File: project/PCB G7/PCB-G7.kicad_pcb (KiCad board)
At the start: 2 copper layers, 56.5 x 88 mm, 28 parts, among them J13 jumper 1 2, J14 jumper 2 2, J15 stepper 1, J16 jumper 2 1, J17 stepper 1, J18 Barrel_Jack_Switch, J19 servomoteur, J2 Micro_SD_Card, J20 Oled, J9 jumper 1 1, U3 ESP32-S3-UNO, U4 R-78E5.0-1.0

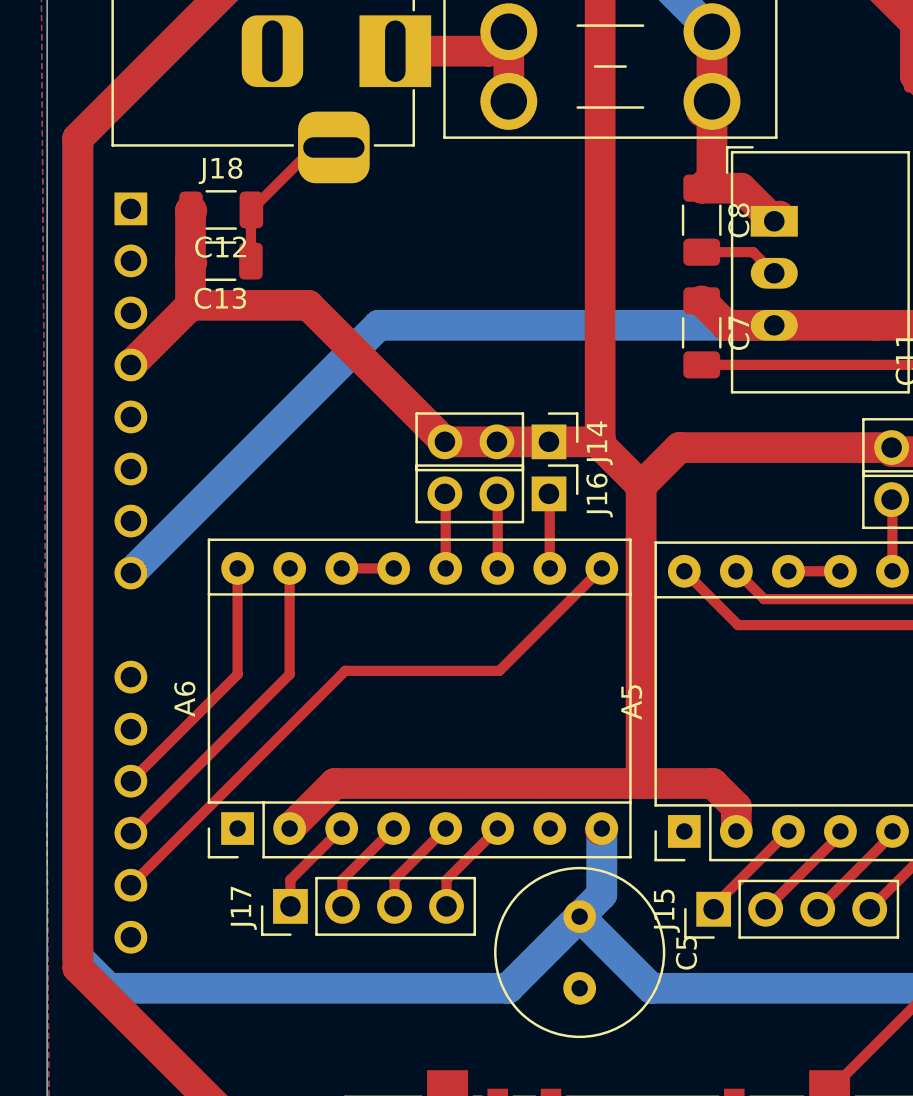
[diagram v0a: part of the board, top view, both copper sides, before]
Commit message: fix some wiring problems
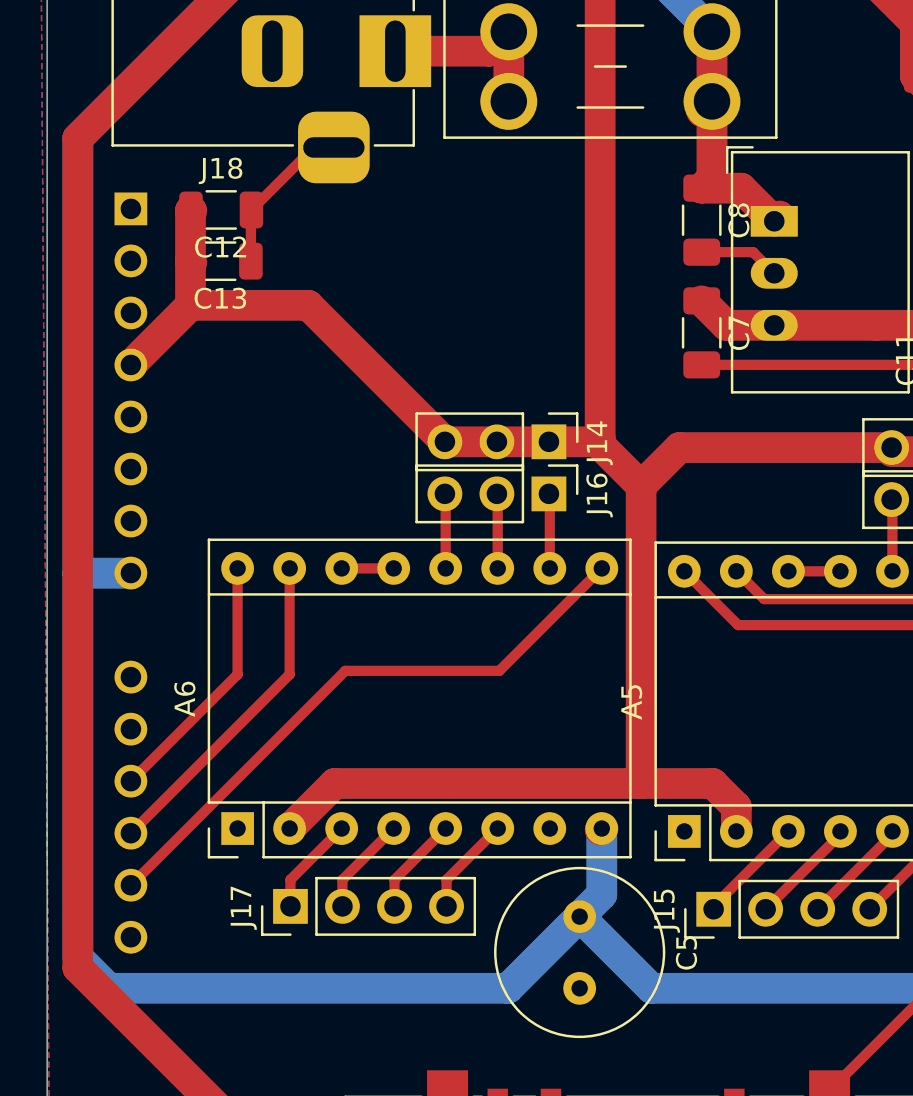
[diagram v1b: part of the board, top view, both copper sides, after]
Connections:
- U3 pad 8: +5V -> +12V
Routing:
- net +5V: track 52.7 -> 16.2 mm
- net +12V: track 149.1 -> 151.7 mm
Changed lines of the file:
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@@
 			(unit
 				(name "A")
-				(pins "20" "19" "1" "3" "9" "10" "11" "12" "13" "14" "5" "2" "7" "6"
-					"29" "4" "8" "16" "15" "30" "32" "31" "28" "27" "26" "25" "24" "23"
-					"22" "21" "18" "17"
+				(pins "20" "19" "1" "3" "9" "10" "11" "12" "13" "14" "5" "2" "6" "29"
+					"7" "4" "8" "16" "15" "30" "32" "31" "28" "27" "26" "25" "24" "23" "22"
+					"21" "18" "17"
 				)
 			)
@@
 			(layers "*.Cu" "*.Mask")
 			(remove_unused_layers no)
-			(net "+5V")
+			(net "+12V")
 			(pinfunction "Vin_8")
 			(pintype "power_in")
@@
 	)
 	(segment
-		(start 136.09 104.7275)
-		(end 148.185 92.6325)
-		(width 1.5)
-		(layer "B.Cu")
-		(net "+5V")
-	)
-	(segment
-		(start 148.185 92.6325)
-		(end 167.5 92.6325)
-		(width 1.5)
-		(layer "B.Cu")
-		(net "+5V")
-	)
-	(segment
 		(start 182.0875 95.5875)
 		(end 184.35 95.5875)
@@
 	(segment
 		(start 133.5 123.5)
-		(end 133.5 83.5)
+		(end 133.5 104.75)
 		(width 1.5)
 		(layer "B.Cu")
@@
 	)
 	(segment
+		(start 133.5 104.75)
+		(end 133.5 83.5)
+		(width 1.5)
+		(layer "B.Cu")
+		(net "+12V")
+	)
+	(segment
 		(start 133.5 83.5)
 		(end 141.5 75.5)
@@
 	)
 	(segment
+		(start 133.5225 104.7275)
+		(end 136.09 104.7275)
+		(width 1.5)
+		(layer "B.Cu")
+		(net "+12V")
+	)
+	(segment
 		(start 154.5 125)
 		(end 135 125)
 		(width 1.5)
 		(layer "B.Cu")
+		(net "+12V")
+	)
+	(segment
+		(start 133.5 104.75)
+		(end 133.5225 104.7275)
+		(width 1.5)
+		(layer "B.Cu")
